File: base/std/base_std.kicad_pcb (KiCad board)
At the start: 2 copper layers, 25.2 x 30 mm, 19 parts, among them J1 Moat_Wire_12, J10 1wireConn, J2 Moat_Bus_wire, J3 I2C, J4 Conn_01x08, Q1 2N7002

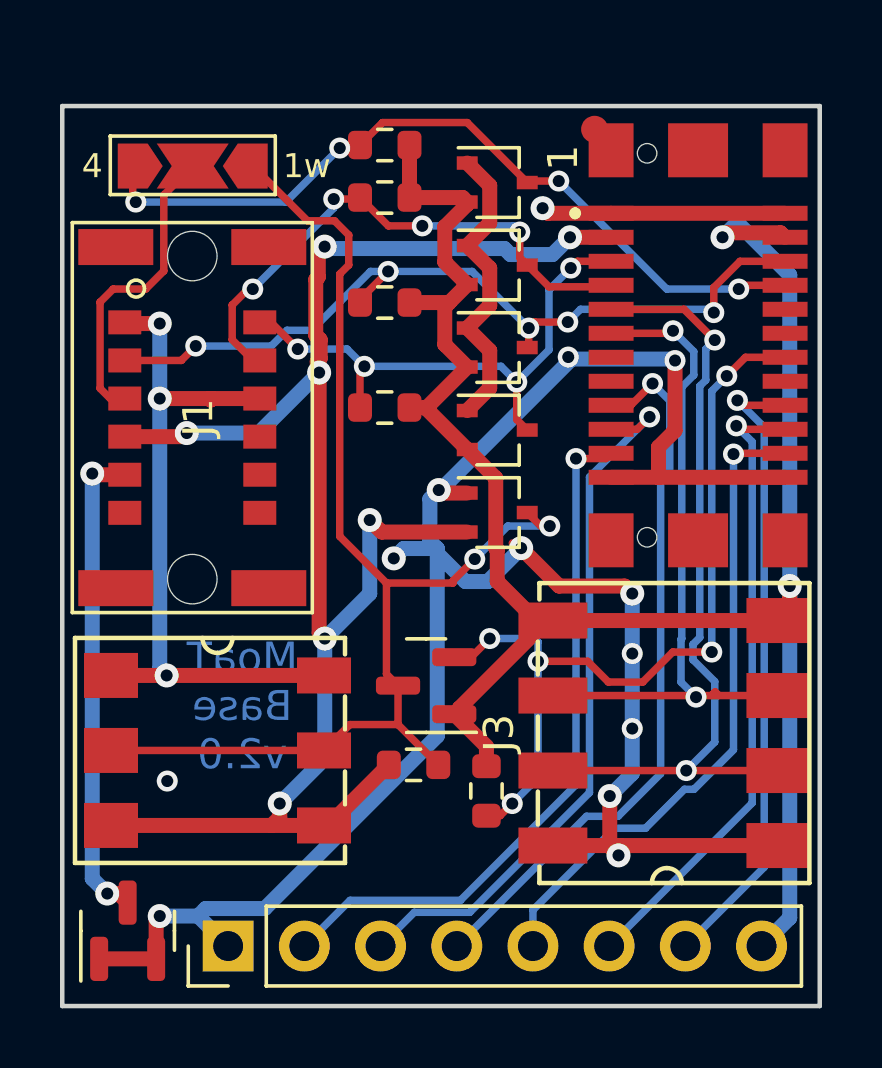
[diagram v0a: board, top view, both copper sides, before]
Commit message: misc updates I didn't bother checking in, oops
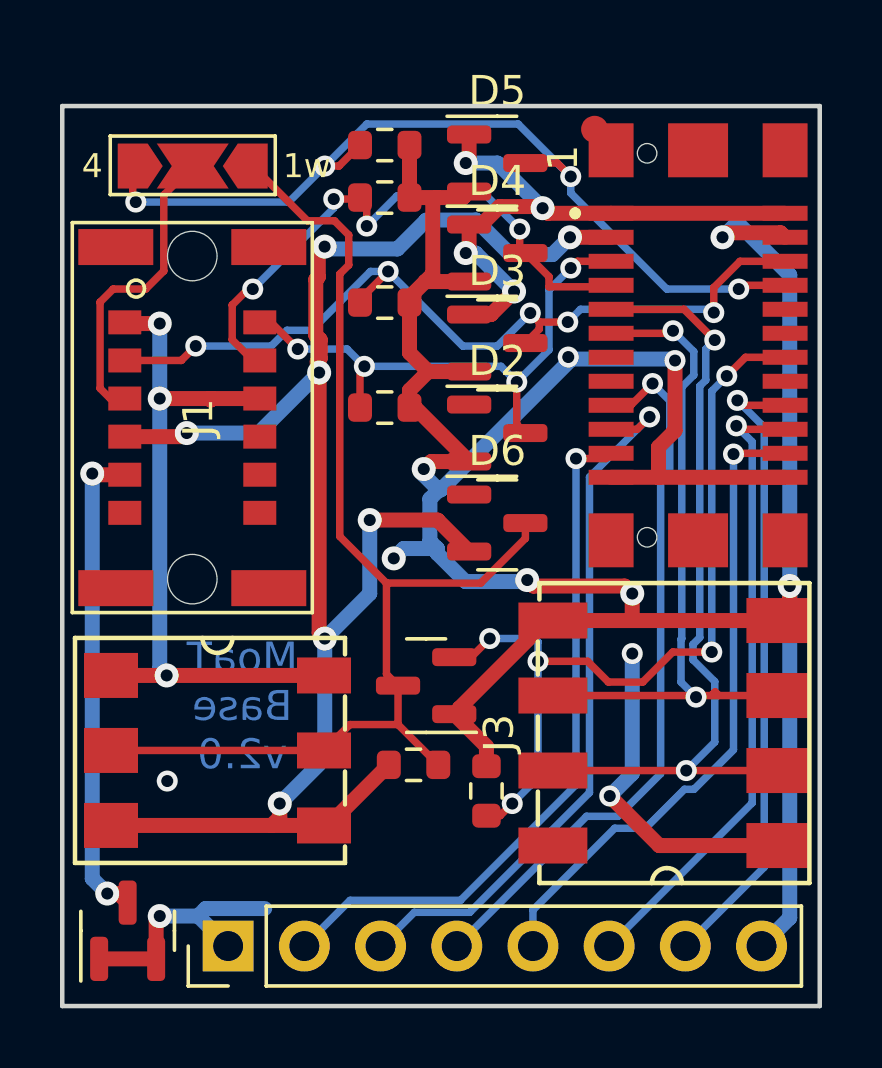
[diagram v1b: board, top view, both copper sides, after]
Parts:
- D2, D3, D4, D5, D6: footprint Package_TO_SOT_SMD:SOT-323_SC-70 -> Package_TO_SOT_SMD:SOT-23
- moved D5 0.65 mm to (37.2, 23.1)
- moved D4 0.40 mm to (37.2, 26.1)
- moved D6 0.35 mm to (37.2, 35.1)
- moved D3 0.15 mm to (37.2, 29.1)
- moved D2 0.10 mm to (37.2, 32.1)
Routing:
- net GND: track 114.4 -> 63.2 mm, vias 16 -> 12
- net +3V3: track 66.6 -> 95.0 mm, vias 2 -> 7
- net /Bus4: track 26.4 -> 29.8 mm
- net /1wire_5: track 40.6 -> 39.0 mm, vias 2 -> 0
- net /Bus3: track 18.4 -> 19.7 mm
- net +5V: track 55.6 -> 56.7 mm
- net /Bus2: track 27.5 -> 28.5 mm
